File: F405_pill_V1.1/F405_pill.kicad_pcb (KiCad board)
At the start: 4 copper layers, 53.8 x 19.4 mm, 42 parts, among them J1 Conn_01x04_Male, J2 Conn_01x04_Male, J4 TYPE-C-31-M-12, U1 STM32F405RGTx, U2 TCAN1051HDR, U3 LM1117-3.3, U4 STM32F405_pill, Y1 Crystal_GND24

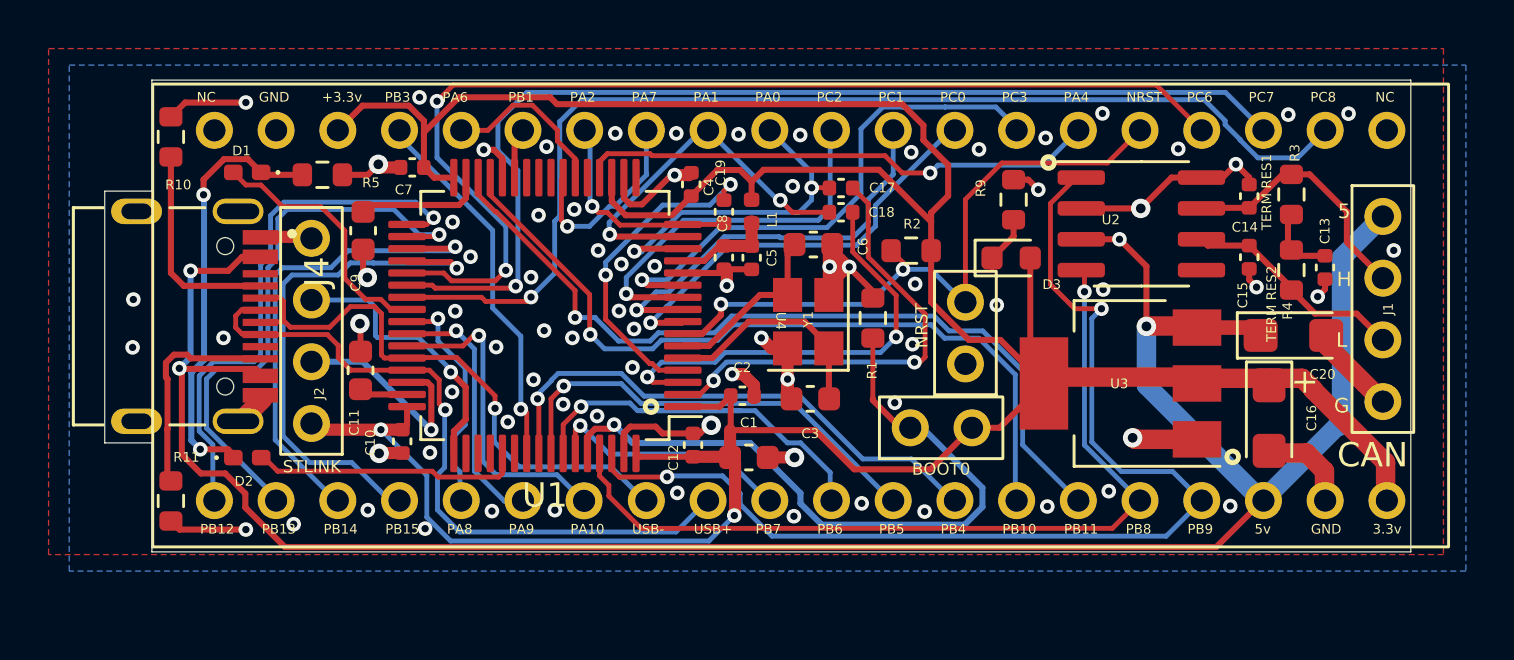
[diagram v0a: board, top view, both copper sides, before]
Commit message: new notes
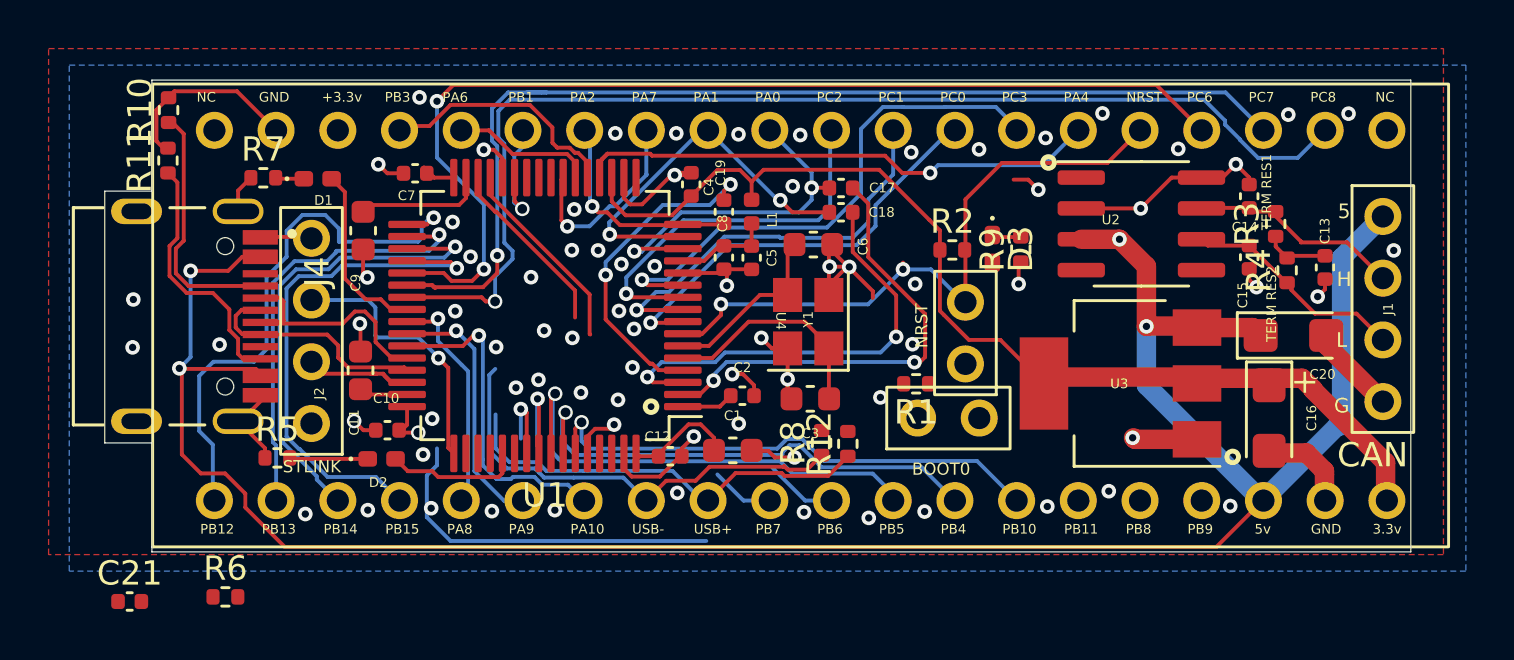
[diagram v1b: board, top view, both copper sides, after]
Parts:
- added C21: ??, Capacitor_SMD:C_0402_1005Metric, F.Cu at (95.4, 96.5)
- added R12: 1k, Resistor_SMD:R_0402_1005Metric, F.Cu at (125.0, 90.0)
- added R6: ??, Resistor_SMD:R_0402_1005Metric, F.Cu at (99.3, 96.3)
- added R7: 20k, Resistor_SMD:R_0402_1005Metric, F.Cu at (100.9, 79.0)
- added R8: 1k, Resistor_SMD:R_0402_1005Metric, F.Cu at (123.9, 89.9)
- D3: footprint LED_SMD:LED_0603_1608Metric -> LED_SMD:LED_0402_1005Metric_Pad0.77x0.64mm_HandSolder
- R1, R10, R11, R2, R3, R4, R9: footprint Resistor_SMD:R_0603_1608Metric -> Resistor_SMD:R_0402_1005Metric
- R5: value 5k -> 20k; footprint Resistor_SMD:R_0603_1608Metric -> Resistor_SMD:R_0402_1005Metric
- moved R11 14.0 mm to (97.0, 78.3), turned to 90 degrees
- moved R5 11.8 mm to (101.5, 90.5), turned to 0 degrees
- moved D2 5.53 mm to (105.8, 90.6)
- moved R1 3.24 mm to (127.8, 87.5), turned to 180 degrees
- moved D1 2.91 mm to (103.1, 79.0), turned to 0 degrees
- moved R9 2.07 mm to (132.1, 82.0), turned to 90 degrees
- moved R2 1.70 mm to (129.3, 82.0), turned to 0 degrees
- moved R3 1.38 mm to (142.6, 80.9)
- moved R10 1.11 mm to (97.0, 76.2)
- moved C12 1.04 mm to (117.7, 90.5), turned to 0 degrees
- moved D3 0.86 mm to (130.9, 81.9), turned to -90 degrees
- moved C10 0.76 mm to (106.0, 89.4), turned to 180 degrees
- moved C1 0.72 mm to (120.2, 90.2)
- moved JP1 0.50 mm to (129.1, 88.9)
- moved C7 0.27 mm to (107.2, 78.8)
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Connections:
- D2 pad 1: Net-(D1-Pad1) -> Net-(D2-Pad1)
- R5 pad 2: Net-(D1-Pad1) -> Net-(D2-Pad1)
- U1 pad 24: PC4 -> DUAL1
- U1 pad 25: PC5 -> DUAL2
- U2 pad 5: GND -> unconnected-(U2-Pad5)
- U4 pad 17: PB3 -> PA5
- U4 pad 28: USB_D- -> DUAL1
- U4 pad 29: USB_D+ -> DUAL2
- U4 pad 30: PB7 -> PB3
- U4 pad 31: PB6 -> PB4
- U4 pad 33: PB4 -> PB6
- U4 pad 34: PB10 -> PB7
- U4 pad 35: PB11 -> PC10
- U4 pad 36: PB8 -> PC11
- U4 pad 37: PB9 -> PC12
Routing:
- net +3V3: track 132.5 -> 70.5 mm
- net PB9: track 45.7 -> 0.00 mm, vias 2 -> 0
- net PB8: track 35.3 -> 0.00 mm, vias 1 -> 0
- net Net-(JP1-Pad2): track 28.8 -> 2.00 mm
- net PB11: track 33.9 -> 7.44 mm, vias 1 -> 0
- net PB10: track 32.4 -> 8.16 mm, vias 1 -> 0
- net USB_D+: track 28.8 -> 9.72 mm, vias 1 -> 0
- net DUAL1: track 0.00 -> 18.9 mm
- net DUAL2: track 0.00 -> 17.6 mm
- net Net-(D1-Pad1): track 17.7 -> 1.17 mm, vias 2 -> 0
- net PB4: track 22.1 -> 7.20 mm
- net USB_D-: track 23.6 -> 10.3 mm, vias 1 -> 0
- net PB7: track 10.3 -> 21.4 mm
- net PA5: track 0.00 -> 10.4 mm
- net PB3: track 15.5 -> 5.81 mm
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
